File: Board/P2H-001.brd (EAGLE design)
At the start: 72 x 72 mm, 26 parts, among them IC1 LTC485N, IC2 74LS07N, IC3 74LS157N, IC4 LTC485N, IC5 TLC5941NT, U1 ARDUINO_PRO_MINI

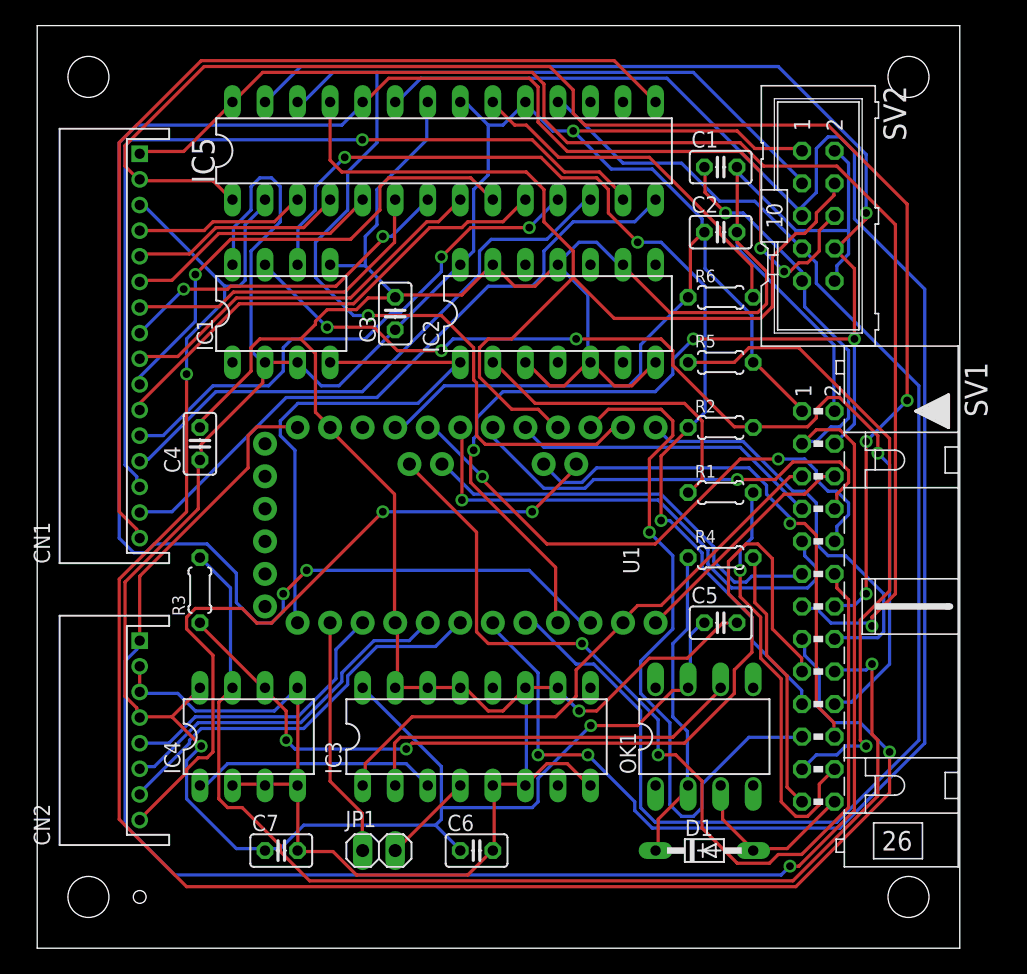
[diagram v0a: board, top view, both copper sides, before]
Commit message: Brush up.
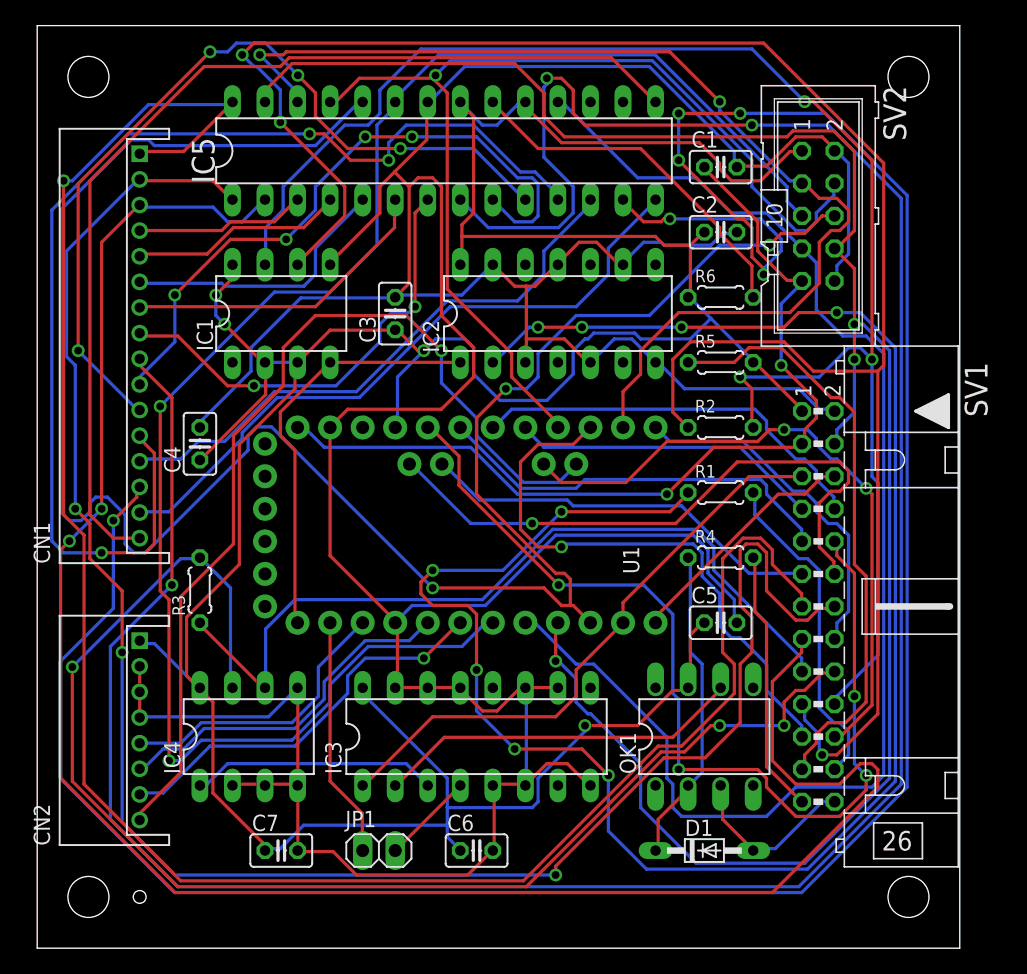
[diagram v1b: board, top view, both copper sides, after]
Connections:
- net GND: now also CN2.4
- net VCC: now also CN2.1; no longer CN2.4
- net VDD: no longer CN2.1
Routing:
- net LED3B: track 30.3 -> 206.3 mm, vias 0 -> 3
- net N$5: track 68.3 -> 198.0 mm, vias 1 -> 6
- net N$2: track 24.3 -> 148.4 mm, vias 0 -> 9
- net VDD: track 162.2 -> 70.9 mm
- net TX+: track 82.3 -> 152.5 mm
- net GND: track 284.5 -> 339.7 mm, vias 1 -> 0
- net N$8: track 42.0 -> 90.8 mm, vias 2 -> 3
- net LEDA: track 106.4 -> 153.7 mm
- net TX-: track 80.9 -> 121.8 mm, vias 4 -> 3
- net A3: track 44.8 -> 76.7 mm, vias 2 -> 4
- net N$12: track 114.8 -> 144.1 mm
- net N$7: track 37.2 -> 65.3 mm, vias 0 -> 4
- net MODE: track 127.5 -> 155.4 mm, vias 4 -> 3
- net A5: track 76.0 -> 48.3 mm, vias 2 -> 1
- net VR: track 56.2 -> 73.7 mm, vias 2 -> 1
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
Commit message: Hotfix.
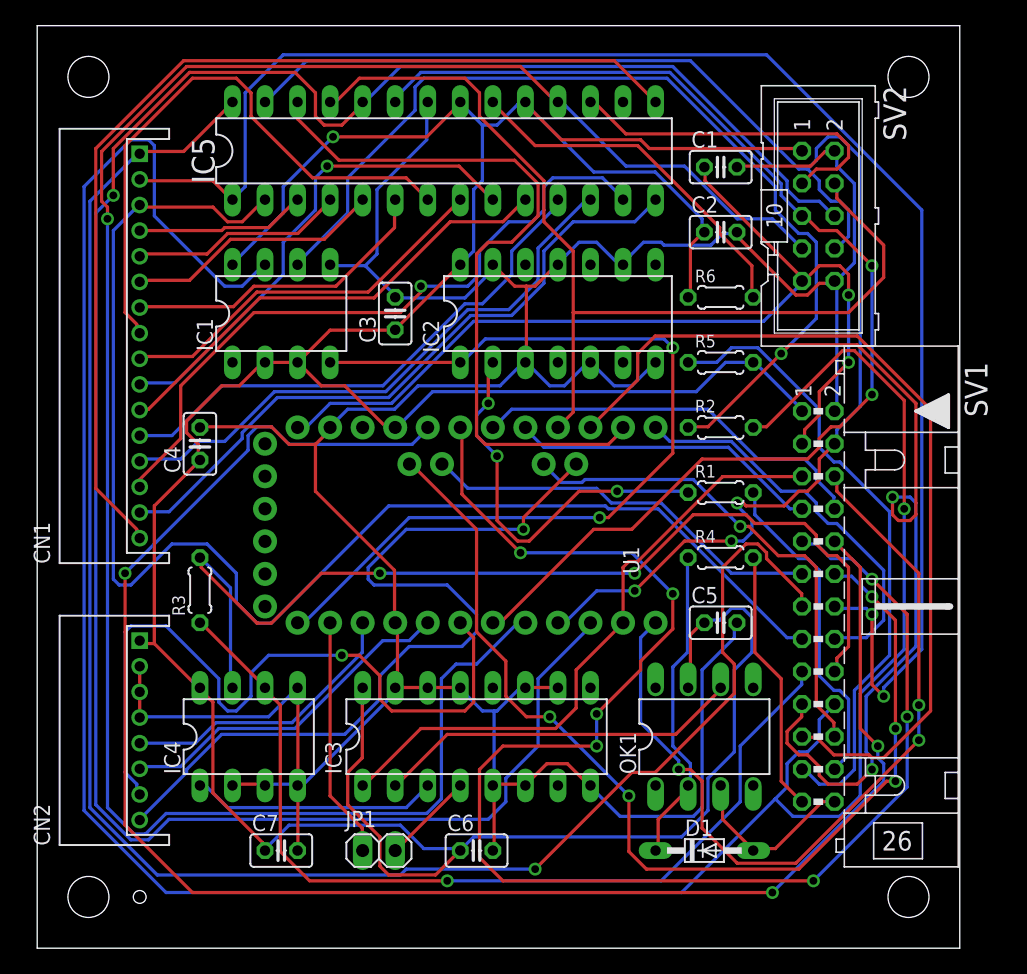
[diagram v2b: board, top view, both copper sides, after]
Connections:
- new net N$10: IC5.17, SV2.3
- net SIN: no longer SV2.3
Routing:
- net LED3B: track 206.3 -> 30.3 mm, vias 3 -> 0
- net N$5: track 198.0 -> 53.6 mm, vias 6 -> 1
- net N$2: track 148.4 -> 30.9 mm, vias 9 -> 3
- net A2: track 31.9 -> 117.2 mm, vias 0 -> 7
- net TX-: track 121.8 -> 198.3 mm, vias 3 -> 1
- net GND: track 339.7 -> 269.9 mm
- net A3: track 76.7 -> 135.1 mm, vias 4 -> 3
- net GSCLCK: track 107.2 -> 160.5 mm, vias 0 -> 1
- net N$8: track 90.8 -> 41.6 mm, vias 3 -> 0
- net GDETECT: track 19.0 -> 64.5 mm, vias 0 -> 3
- net N$14: track 151.0 -> 108.5 mm, vias 2 -> 0
- net BLANK: track 131.9 -> 92.7 mm
- net MODE: track 155.4 -> 116.7 mm
- net TX: track 32.6 -> 70.9 mm, vias 0 -> 2
- net A5: track 48.3 -> 81.5 mm, vias 1 -> 5
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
